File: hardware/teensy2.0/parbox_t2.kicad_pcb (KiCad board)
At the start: 2 copper layers, 49.8 x 41.9 mm, 17 parts, among them J1 DB25_Male, J2 Debug Header, J3 I2C OLED, J4 I2C Extra, J5 ENC28J60 Module, J6 NET Select, J7 SD Card Breakout, J8 EN_EXT_INT, J9 AVR ISP, U1 Teensy2.0_(C), U2 WIZ820IO, U3 LM1117-3.3

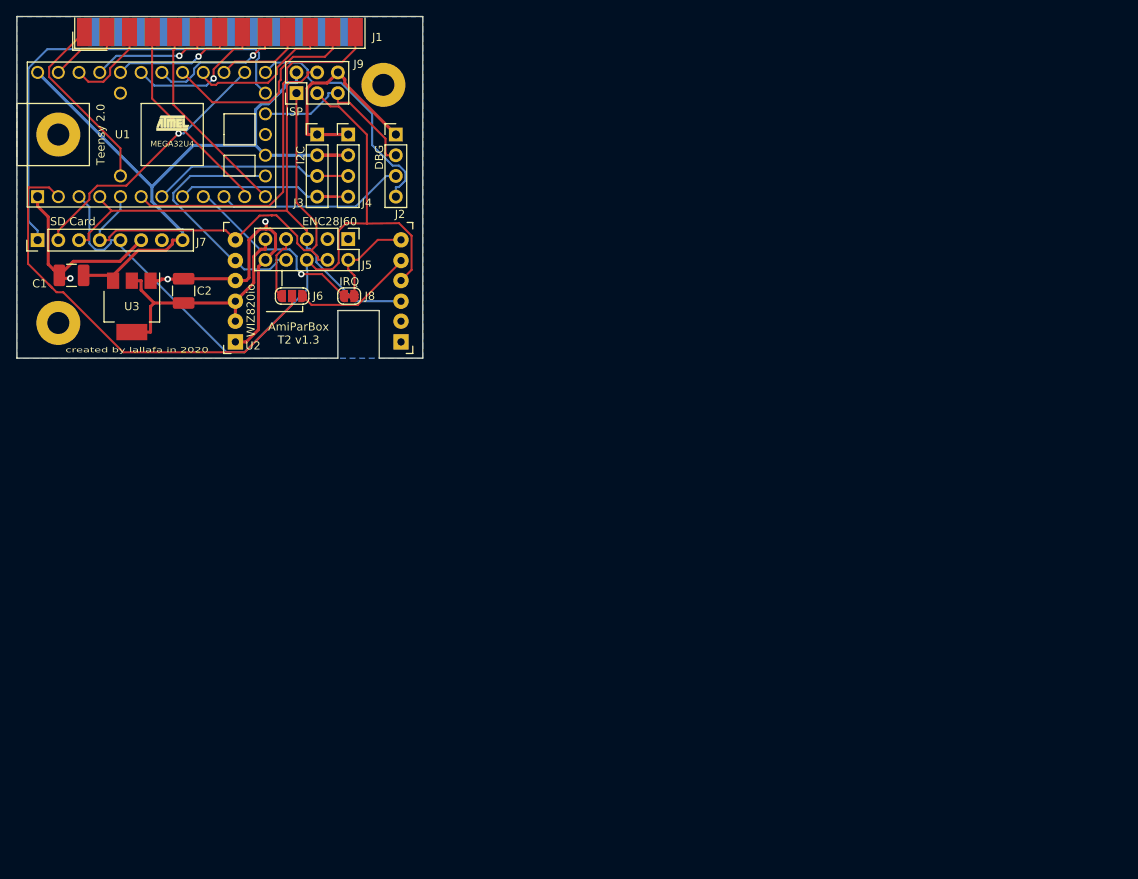
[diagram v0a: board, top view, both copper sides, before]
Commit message: hw: update t2 rev 1.4
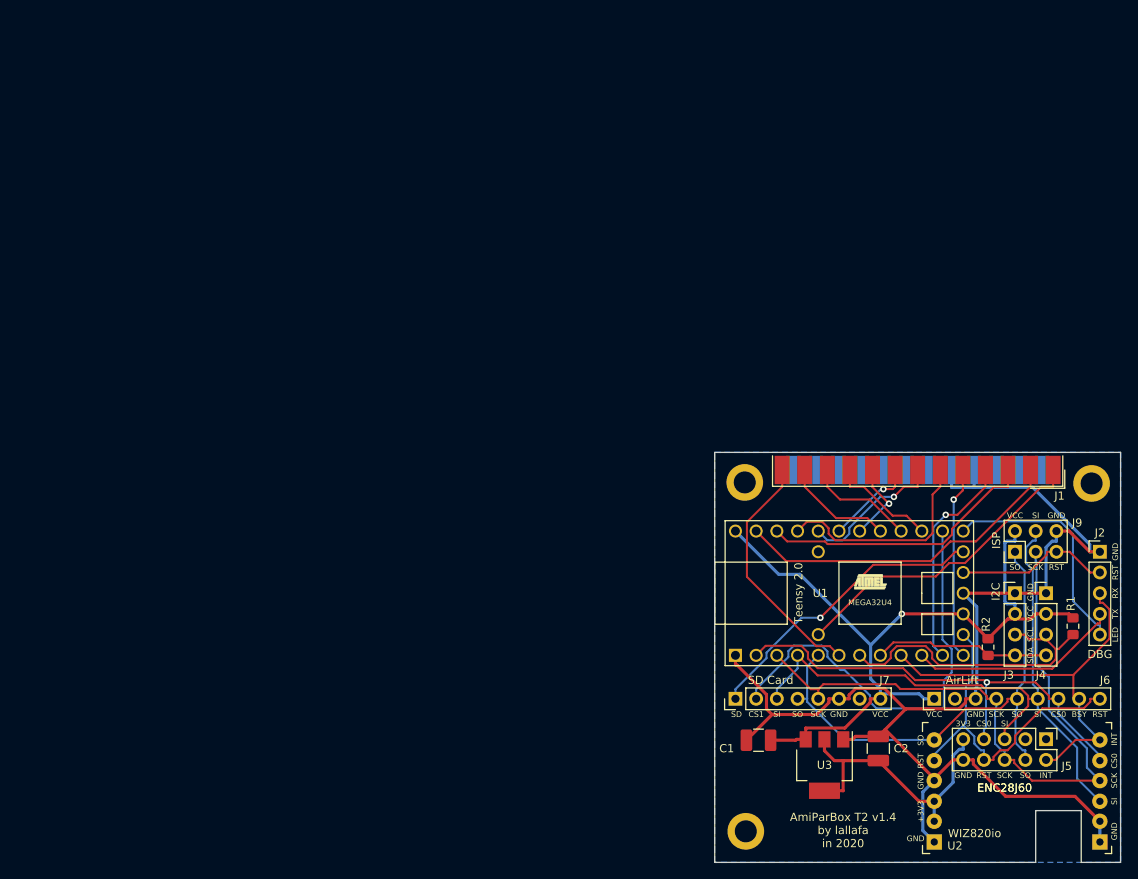
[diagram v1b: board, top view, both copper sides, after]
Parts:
- removed J8: EN_EXT_INT, Jumper:SolderJumper-2_P1.3mm_Bridged_RoundedPad1.0x1.5mm
- added R1: 4k7, Resistor_SMD:R_0805_2012Metric_Pad1.15x1.40mm_HandSolder, F.Cu at (164.3, 102.7)
- added R2: 4k7, Resistor_SMD:R_0805_2012Metric_Pad1.15x1.40mm_HandSolder, F.Cu at (153.9, 105.3)
- H1, H2, H3: footprint MountingHole:MountingHole_2.7mm_M2.5_Pad -> MountingHole:MountingHole_2.7mm_M2.5_ISO14580_Pad
- J1: footprint modules:DSUB-25_Female_EdgeMount_P2.77mm -> modules:DSUB-25_Male_EdgeMount_P2.77mm
- J2: value Debug Header -> Debug; footprint Connector_PinHeader_2.54mm:PinHeader_1x04_P2.54mm_Vertical -> Connector_PinHeader_2.54mm:PinHeader_1x05_P2.54mm_Vertical
- J6: value NET Select -> ESP32 AirLift; footprint Jumper:SolderJumper-3_P1.3mm_Open_RoundedPad1.0x1.5mm_NumberLabels -> Connector_PinHeader_2.54mm:PinHeader_1x09_P2.54mm_Vertical
- moved U2 105.4 mm to (157.5, 122.9)
- moved J5 105.3 mm to (161.0, 116.6)
- moved H1 104.9 mm to (124.2, 127.9)
- moved J9 104.6 mm to (157.2, 93.6)
- moved J3 102.4 mm to (161.0, 98.7)
- moved J4 102.4 mm to (157.2, 98.7)
- moved J7 102.4 mm to (122.9, 111.6)
- moved U1 102.4 mm to (136.9, 98.7)
- moved C2 102.0 mm to (140.5, 117.7)
- moved U3 101.9 mm to (133.9, 119.8)
- moved C1 101.8 mm to (125.8, 116.7)
- moved J1 101.1 mm to (145.3, 83.6)
- moved J2 100.4 mm to (167.6, 93.6)
- moved H2 99.7 mm to (166.6, 85.2)
- moved H3 94.4 mm to (124.1, 85.1)
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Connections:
- J2 pad 3: /TXD -> /EXT_INT
- J2 pad 4: /LED -> /TXD
- J5 pad 2: /EN_INT -> /EXT_INT
- J5 pad 7: /SS_ENC -> /SS0
- J6 pad 1: /SS_WIZ -> VCC
- J6 pad 2: /SS0 -> Net-(J6-Pad2)
- J6 pad 3: /SS_ENC -> GND
- U2 pad J1-5: /SS_WIZ -> /SS0
- U2 pad J1-6: /EN_INT -> /EXT_INT
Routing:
- net GND: track 90.0 -> 185.1 mm, vias 3 -> 0
- net /DATA0: track 9.22 -> 41.0 mm
- net /EXT_INT: track 23.2 -> 52.0 mm, vias 1 -> 0
- net /DATA1: track 10.9 -> 34.4 mm
- net /SS1: track 32.5 -> 53.4 mm, vias 1 -> 0
- net /SD_DETECT: track 56.5 -> 36.5 mm, vias 0 -> 1
- net /STROBE: track 23.1 -> 38.4 mm
- net /SEL: track 45.4 -> 30.2 mm
- net /SS_WIZ: track 14.8 -> 0.00 mm
- net /POUT: track 26.3 -> 13.6 mm
- net /EN_INT: track 12.3 -> 0.00 mm
- net /MOSI: track 70.2 -> 82.0 mm
- net /DATA4: track 15.2 -> 26.9 mm, vias 1 -> 0
- net VCC: track 83.7 -> 95.1 mm, vias 0 -> 1
- net /SCL: track 26.9 -> 38.0 mm
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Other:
- board size 49.8 x 41.9 mm -> 49.8 x 50.3 mm
- board text added: "+3V3"
- board text added: "3V3"
- board text added: "AirLift"
- board text added: "AmiParBox T2 v1.4 by lallafa in 2020"
- board text added: "BSY"
- board text added: "CS0"
- board text added: "CS1"
- board text added: "GND"
- board text added: "INT"
- board text added: "LED"
- board text added: "RST"
- board text added: "RX"
- board text added: "SCK"
- board text added: "SCL"
- board text added: "SD"
- board text added: "SDA"
- board text added: "SI"
- board text added: "SO"
- board text added: "TX"
- board text added: "VCC"
- board text removed: "AmiParBox T2 v1.3"
- board text removed: "IRQ"
- board text removed: "created by lallafa in 2020"
